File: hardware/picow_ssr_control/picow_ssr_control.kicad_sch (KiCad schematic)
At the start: 6 parts

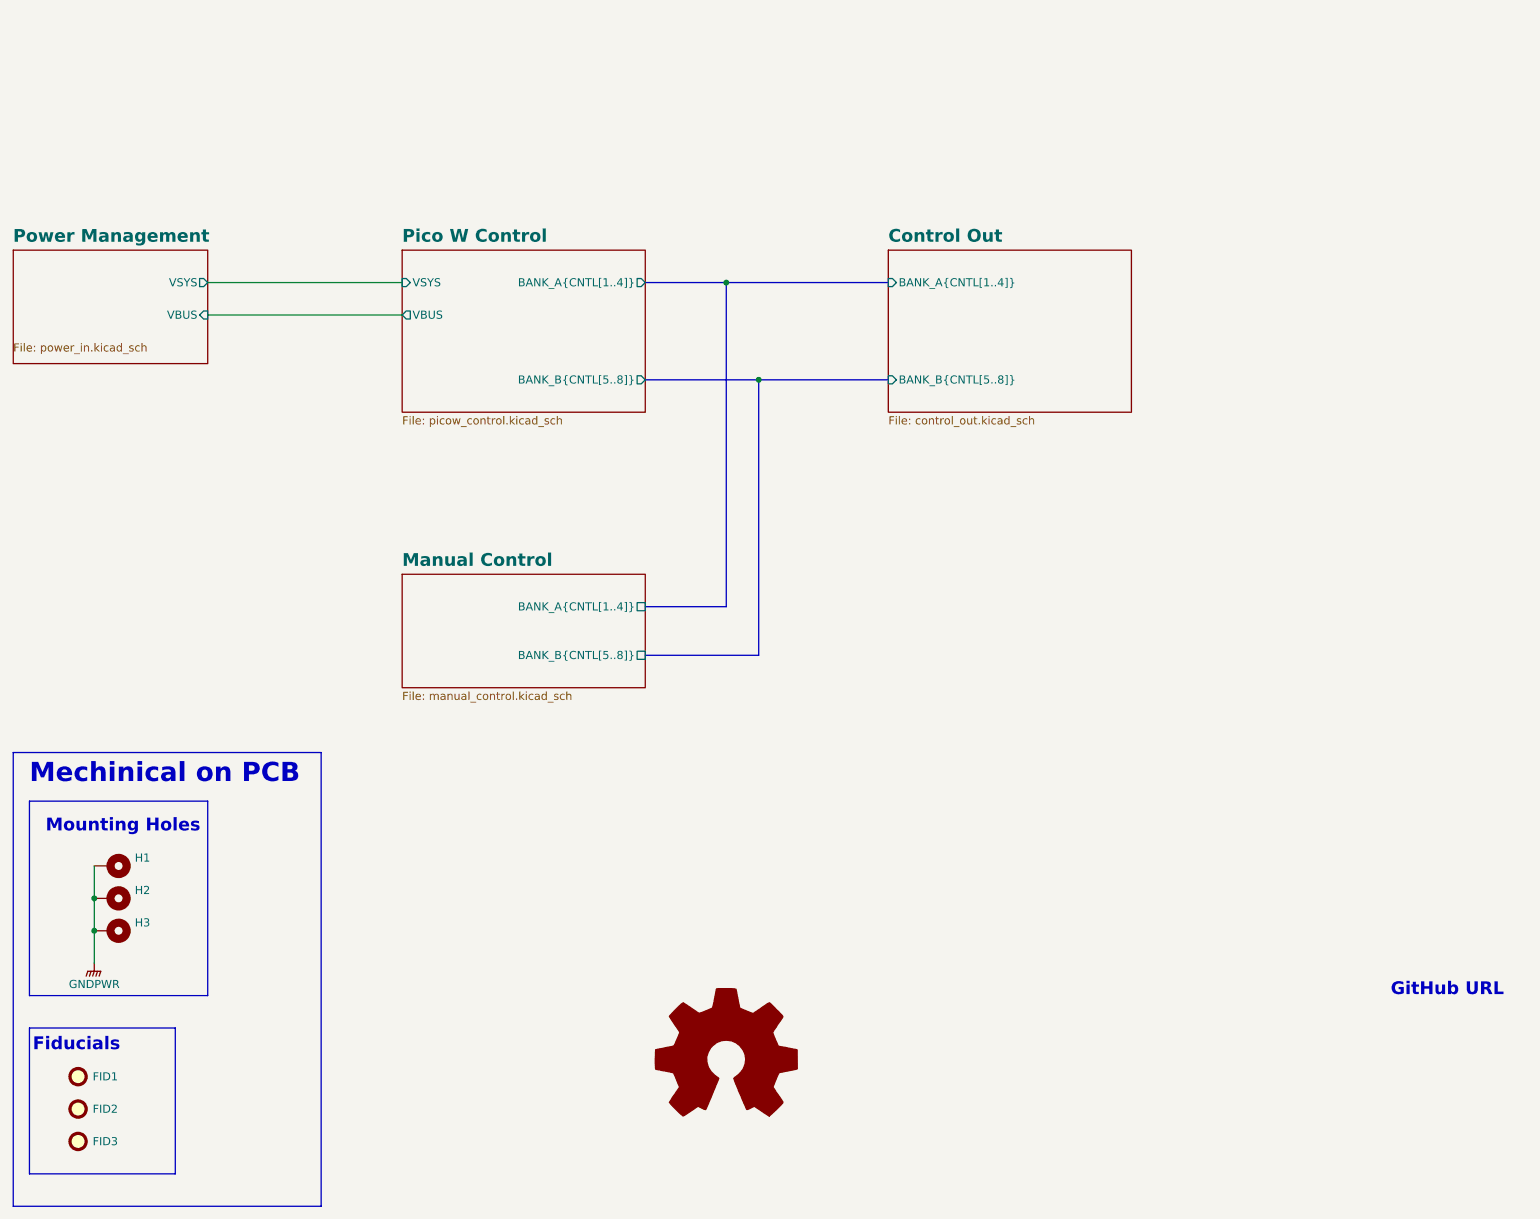
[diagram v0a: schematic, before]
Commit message: Updated schemas
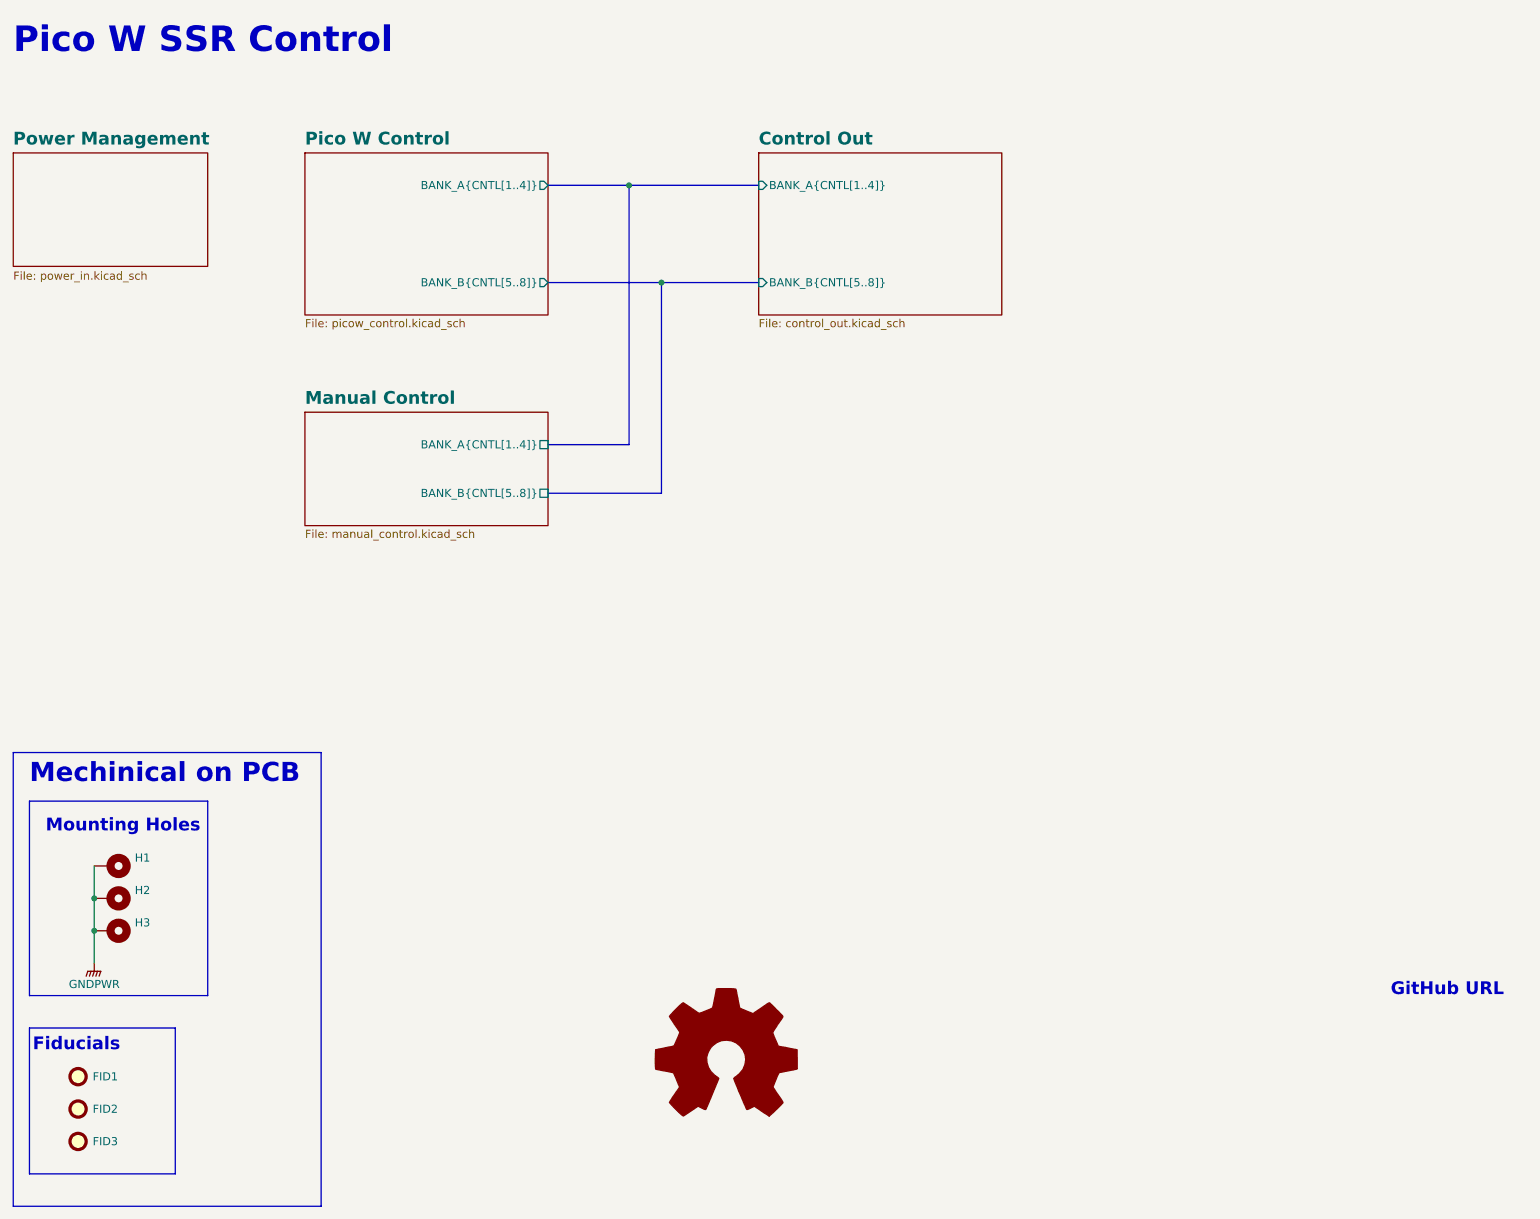
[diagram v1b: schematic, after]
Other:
- sheet Pico W Control ports: added none; removed VBUS, VSYS
- sheet Power Management ports: added none; removed VBUS, VSYS
- note added: "Pico W SSR Control"
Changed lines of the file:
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@@
   (title_block
     (title "Picow SSR Control")
-    (date "2023-01-27")
+    (date "2023-01-28")
     (rev "0.0.10")
     (comment 2 "http://creativecommons.org/licenses/by-sa/4.0/")
@@
     (comment 6 "Hardware License: CERN-OHL-W")
   )
-  (junction (at 127 55.88) (diameter 0) (color 255 255 0 1)
+  (junction (at 111.76 40.64) (diameter 0) (color 255 255 0 1)
   )
   (junction (at 27.94 152.4) (diameter 0) (color 0 0 0 0)
@@
   (junction (at 27.94 157.48) (diameter 0) (color 0 0 0 0)
   )
-  (junction (at 132.08 71.12) (diameter 0) (color 255 255 0 1)
+  (junction (at 116.84 55.88) (diameter 0) (color 255 255 0 1)
   )
   (polyline (pts (xy 17.78 172.72) (xy 17.78 195.58))
@@
     (stroke (width 0) (type default) (color 0 0 0 0))
   )
-  (bus (pts (xy 127 55.88) (xy 127 106.68))
+  (bus (pts (xy 111.76 40.64) (xy 111.76 81.28))
     (stroke (width 0) (type default) (color 255 255 0 1))
   )
@@
     (stroke (width 0) (type default) (color 0 0 0 0))
   )
-  (bus (pts (xy 132.08 71.12) (xy 152.4 71.12))
+  (bus (pts (xy 116.84 55.88) (xy 132.08 55.88))
     (stroke (width 0) (type default) (color 255 255 0 1))
   )
@@
     (stroke (width 0) (type default) (color 0 0 0 0))
   )
-  (bus (pts (xy 127 55.88) (xy 152.4 55.88))
+  (bus (pts (xy 111.76 40.64) (xy 132.08 40.64))
     (stroke (width 0) (type default) (color 255 255 0 1))
   )
@@
     (stroke (width 0) (type default) (color 0 0 0 0))
   )
-  (bus (pts (xy 132.08 114.3) (xy 114.3 114.3))
+  (bus (pts (xy 116.84 88.9) (xy 99.06 88.9))
     (stroke (width 0) (type default) (color 255 255 0 1))
   )
@@
     (stroke (width 0) (type default) (color 0 0 0 0))
   )
-  (wire (pts (xy 45.72 55.88) (xy 76.2 55.88))
-    (stroke (width 0) (type default) (color 0 0 0 0))
-  )
   (wire (pts (xy 27.94 152.4) (xy 27.94 157.48))
     (stroke (width 0) (type default) (color 0 0 0 0))
   )
-  (bus (pts (xy 114.3 106.68) (xy 127 106.68))
+  (bus (pts (xy 99.06 81.28) (xy 111.76 81.28))
     (stroke (width 0) (type default) (color 255 255 0 1))
   )
@@
     (stroke (width 0) (type default) (color 0 0 0 0))
   )
-  (bus (pts (xy 132.08 71.12) (xy 132.08 114.3))
+  (bus (pts (xy 116.84 55.88) (xy 116.84 88.9))
     (stroke (width 0) (type default) (color 255 255 0 1))
   )
-  (bus (pts (xy 114.3 71.12) (xy 132.08 71.12))
+  (bus (pts (xy 99.06 55.88) (xy 116.84 55.88))
     (stroke (width 0) (type default) (color 255 255 0 1))
   )
-  (wire (pts (xy 45.72 60.96) (xy 76.2 60.96))
-    (stroke (width 0) (type default) (color 0 0 194 1))
-  )
-  (bus (pts (xy 114.3 55.88) (xy 127 55.88))
+  (bus (pts (xy 99.06 40.64) (xy 111.76 40.64))
     (stroke (width 0) (type default) (color 255 255 0 1))
   )
@@
     )
   )
+  (text "Pico W SSR Control" (at 15.24 20.32 0)
+    (effects (font (size 4 4) bold) (justify left bottom))
+  )
   (text "Mounting Holes" (at 20.32 142.24 0)
     (effects (font (size 2 2) (thickness 0.4) bold) (justify left bottom))
@@
     )
   )
-  (sheet (at 76.2 101.6) (size 38.1 17.78) (fields_autoplaced)
+  (sheet (at 60.96 76.2) (size 38.1 17.78) (fields_autoplaced)
     (stroke (width 0.1524) (type solid) (color 0 0 0 0))
     (fill (color 0 0 0 0.0000))
-    (property "Sheet name" "Manual Control" (id 0) (at 76.2 100.5234 0)
+    (property "Sheet name" "Manual Control" (id 0) (at 60.96 75.1234 0)
       (effects (font (size 2 2) bold) (justify left bottom))
     )
-    (property "Sheet file" "manual_control.kicad_sch" (id 1) (at 76.2 119.9646 0)
+    (property "Sheet file" "manual_control.kicad_sch" (id 1) (at 60.96 94.5646 0)
       (effects (font (size 1.27 1.27)) (justify left top))
     )
-    (pin "BANK_A{CNTL[1..4]}" passive (at 114.3 106.68 0)
+    (pin "BANK_A{CNTL[1..4]}" passive (at 99.06 81.28 0)
       (effects (font (size 1.27 1.27)) (justify right))
     )
-    (pin "BANK_B{CNTL[5..8]}" passive (at 114.3 114.3 0)
+    (pin "BANK_B{CNTL[5..8]}" passive (at 99.06 88.9 0)
       (effects (font (size 1.27 1.27)) (justify right))
     )
   )
-  (sheet (at 152.4 50.8) (size 38.1 25.4) (fields_autoplaced)
+  (sheet (at 132.08 35.56) (size 38.1 25.4) (fields_autoplaced)
     (stroke (width 0.1524) (type solid) (color 0 0 0 0))
     (fill (color 0 0 0 0.0000))
-    (property "Sheet name" "Control Out" (id 0) (at 152.4 49.7234 0)
+    (property "Sheet name" "Control Out" (id 0) (at 132.08 34.4834 0)
       (effects (font (size 2 2) bold) (justify left bottom))
     )
-    (property "Sheet file" "control_out.kicad_sch" (id 1) (at 152.4 76.7846 0)
+    (property "Sheet file" "control_out.kicad_sch" (id 1) (at 132.08 61.5446 0)
       (effects (font (size 1.27 1.27)) (justify left top))
     )
-    (pin "BANK_B{CNTL[5..8]}" input (at 152.4 71.12 180)
+    (pin "BANK_B{CNTL[5..8]}" input (at 132.08 55.88 180)
       (effects (font (size 1.27 1.27)) (justify left))
     )
-    (pin "BANK_A{CNTL[1..4]}" input (at 152.4 55.88 180)
+    (pin "BANK_A{CNTL[1..4]}" input (at 132.08 40.64 180)
       (effects (font (size 1.27 1.27)) (justify left))
     )
   )
-  (sheet (at 15.24 50.8) (size 30.48 17.78)
+  (sheet (at 15.24 35.56) (size 30.48 17.78)
     (stroke (width 0.1524) (type solid) (color 0 0 0 0))
     (fill (color 0 0 0 0.0000))
-    (property "Sheet name" "Power Management" (id 0) (at 15.21 49.73 0)
+    (property "Sheet name" "Power Management" (id 0) (at 15.21 34.49 0)
       (effects (font (size 2 2) bold) (justify left bottom))
     )
-    (property "Sheet file" "power_in.kicad_sch" (id 1) (at 15.24 65.3546 0)
+    (property "Sheet file" "power_in.kicad_sch" (id 1) (at 15.24 54.102 0)
       (effects (font (size 1.27 1.27)) (justify left top))
     )
-    (pin "VBUS" input (at 45.72 60.96 0)
-      (effects (font (size 1.27 1.27)) (justify right))
-    )
-    (pin "VSYS" output (at 45.72 55.88 0)
-      (effects (font (size 1.27 1.27)) (justify right))
-    )
-  )
-  (sheet (at 76.2 50.8) (size 38.1 25.4) (fields_autoplaced)
+  )
+  (sheet (at 60.96 35.56) (size 38.1 25.4) (fields_autoplaced)
     (stroke (width 0.1524) (type solid) (color 0 0 0 0))
     (fill (color 0 0 0 0.0000))
-    (property "Sheet name" "Pico W Control" (id 0) (at 76.2 49.7234 0)
+    (property "Sheet name" "Pico W Control" (id 0) (at 60.96 34.4834 0)
       (effects (font (size 2 2) bold) (justify left bottom))
     )
-    (property "Sheet file" "picow_control.kicad_sch" (id 1) (at 76.2 76.7846 0)
+    (property "Sheet file" "picow_control.kicad_sch" (id 1) (at 60.96 61.5446 0)
       (effects (font (size 1.27 1.27)) (justify left top))
     )
-    (pin "VSYS" input (at 76.2 55.88 180)
-      (effects (font (size 1.27 1.27)) (justify left))
-    )
-    (pin "VBUS" output (at 76.2 60.96 180)
-      (effects (font (size 1.27 1.27)) (justify left))
-    )
-    (pin "BANK_B{CNTL[5..8]}" output (at 114.3 71.12 0)
+    (pin "BANK_B{CNTL[5..8]}" output (at 99.06 55.88 0)
       (effects (font (size 1.27 1.27)) (justify right))
     )
-    (pin "BANK_A{CNTL[1..4]}" output (at 114.3 55.88 0)
+    (pin "BANK_A{CNTL[1..4]}" output (at 99.06 40.64 0)
       (effects (font (size 1.27 1.27)) (justify right))
     )
@@
       (reference "#PWR02") (unit 1) (value "GNDPWR") (footprint "")
     )
-    (path "/a7cfd456-3e8b-4e3a-9dc2-46f9e2f2d504/629605ae-093c-4e6d-899a-88d1584af921"
-      (reference "#PWR03") (unit 1) (value "+VDC") (footprint "")
+    (path "/e73b6763-033f-46e1-9aa1-1a9dd8951104/9b96088d-8927-4eed-a676-8c97a42df7c3"
+      (reference "#PWR03") (unit 1) (value "+5V") (footprint "")
     )
     (path "/a7cfd456-3e8b-4e3a-9dc2-46f9e2f2d504/e82ef186-d0ca-4236-82f0-31dacbf8334b"
@@
       (reference "#PWR08") (unit 1) (value "GNDPWR") (footprint "")
     )
+    (path "/e73b6763-033f-46e1-9aa1-1a9dd8951104/a1f016ef-c56d-4024-a5c2-bbf8628338e8"
+      (reference "#PWR09") (unit 1) (value "GNDPWR") (footprint "")
+    )
     (path "/9a31bd8a-9f6c-42a4-99bd-41703d57702f/772ba637-5c96-463c-a7e9-f497978fe28b"
       (reference "#PWR011") (unit 1) (value "GNDPWR") (footprint "")
@@
       (reference "C2") (unit 1) (value "100n") (footprint "Capacitor_SMD:C_0805_2012Metric")
     )
+    (path "/e73b6763-033f-46e1-9aa1-1a9dd8951104/bbf39d05-6c1b-4fb4-8b43-6cae4cd26d1a"
+      (reference "C3") (unit 1) (value "100n") (footprint "Capacitor_SMD:C_0805_2012Metric")
+    )
     (path "/f53b3346-3cf3-4e8a-a8f1-2752a8de3dda"
       (reference "FID1") (unit 1) (value "Fiducial") (footprint "Fiducial:Fiducial_0.5mm_Mask1mm")
@@
       (reference "Q1") (unit 1) (value "IRF4905PBF") (footprint "dragon_mobile:TO254P469X1042X1967-3P")
     )
-    (path "/a7cfd456-3e8b-4e3a-9dc2-46f9e2f2d504/0aaa2676-a0f6-441f-b4d2-d7dc39aa23a7"
-      (reference "Q2") (unit 1) (value "DMG2301L") (footprint "Package_TO_SOT_SMD:SOT-23")
+    (path "/e73b6763-033f-46e1-9aa1-1a9dd8951104/eebbe18a-7277-4977-b24b-8f1e8d50465e"
+      (reference "Q2") (unit 1) (value "DMG2305UX-7") (footprint "Package_TO_SOT_SMD:SOT-23")
     )
     (path "/e73b6763-033f-46e1-9aa1-1a9dd8951104/d899e107-a7e2-42d6-b04f-38deada1b33f"
@@
     )
     (path "/a7cfd456-3e8b-4e3a-9dc2-46f9e2f2d504/ad138bad-9bd6-4294-a36b-690f0cb15cb6"
-      (reference "REG1") (unit 1) (value "LM7805") (footprint "SOT230P700X180-4N")
+      (reference "REG1") (unit 1) (value "LM7805") (footprint "Package_TO_SOT_SMD:SOT-223")
     )
     (path "/a7cfd456-3e8b-4e3a-9dc2-46f9e2f2d504/09d3304d-431b-4b30-adf2-e3fc27b505b4"
@@
     )
     (path "/a7cfd456-3e8b-4e3a-9dc2-46f9e2f2d504/102251af-7d71-4271-be1e-7c08e53df276"
-      (reference "RZ1") (unit 1) (value "100k") (footprint "Resistor_SMD:R_0805_2012Metric")
+      (reference "RZ1") (unit 1) (value "100k") (footprint "Resistor_SMD:R_0603_1608Metric")
     )
     (path "/6f32e7f5-0a22-4bb9-a836-1e48dd69b48f/8f786c38-4138-4f6b-b98d-ec240583ea11"
